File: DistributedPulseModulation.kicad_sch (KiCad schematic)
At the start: 44 parts, among them J1 Conn_02x12_Odd_Even, J2 Conn_02x05_Odd_Even, U1 74LS251, U10 4053, U11 4053, U12 4053, U2 74LVC2G74, U25 74LS85, U28 74LS85, U31 74LS85, U4 MCP23017_SP, U7 4053, U8 4040, U9 4040

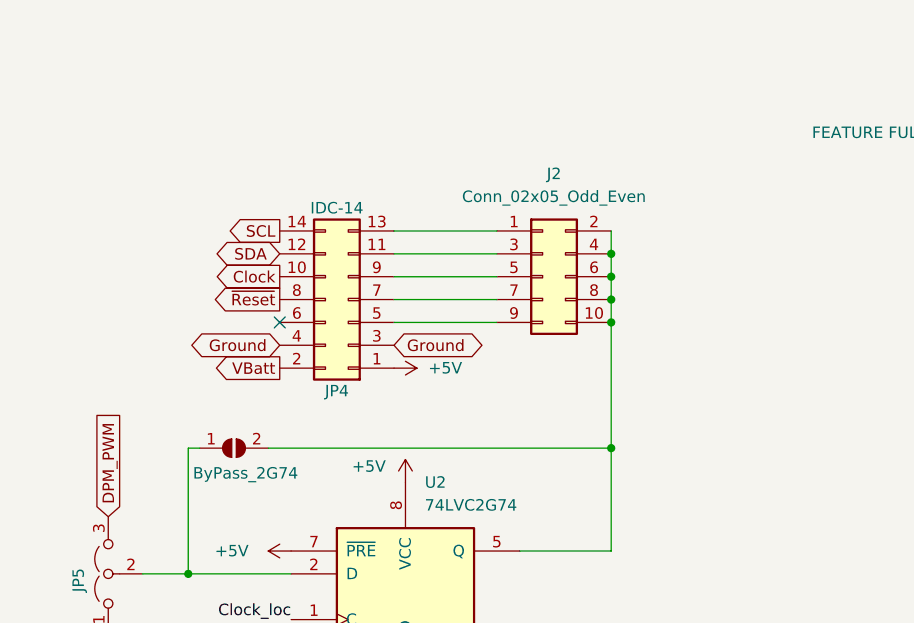
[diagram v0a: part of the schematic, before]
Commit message: Pré-version de la v2.0
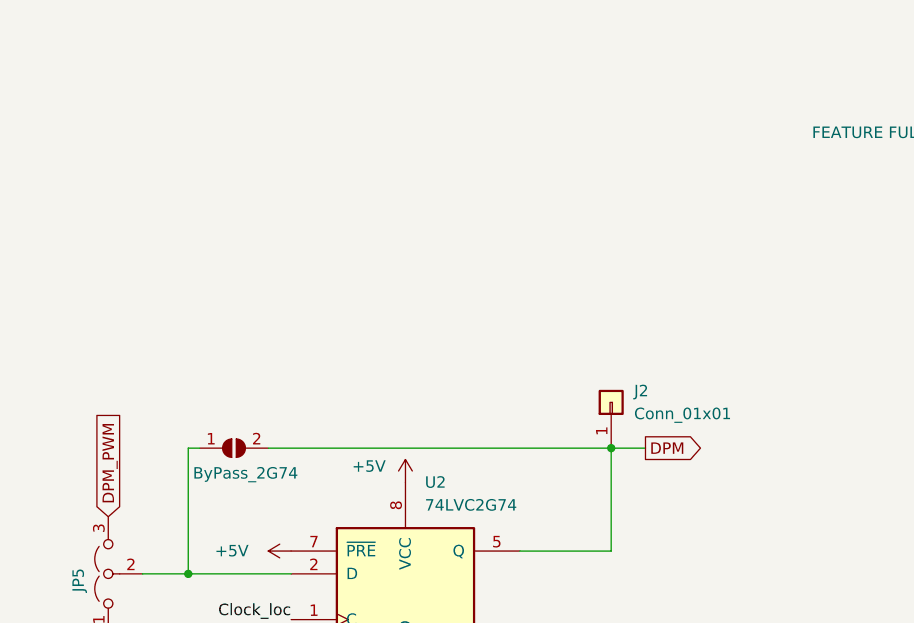
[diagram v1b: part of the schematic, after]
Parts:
- removed J2: Conn_02x05_Odd_Even, Connector_PinHeader_2.54mm:PinHeader_2x05_P2.54mm_Vertical, symbol Connector_Generic:Conn_02x05_Odd_Even
- removed JP4: IDC-14, Connector_IDC:IDC-Header_2x07_P2.54mm_Horizontal, symbol Connector_Generic:Conn_02x07_Odd_Even
- added J2: Conn_01x01, Connector_PinSocket_2.54mm:PinSocket_1x01_P2.54mm_Horizontal, symbol Connector_Generic:Conn_01x01
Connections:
- net DPM: now reaches ByPass_2G74.2 (B), U2.5 (Q)
- net DPM: now also J2.1 (Pin_1)
- no-connect marks 27 -> 26
